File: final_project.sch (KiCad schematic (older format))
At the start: 0 parts

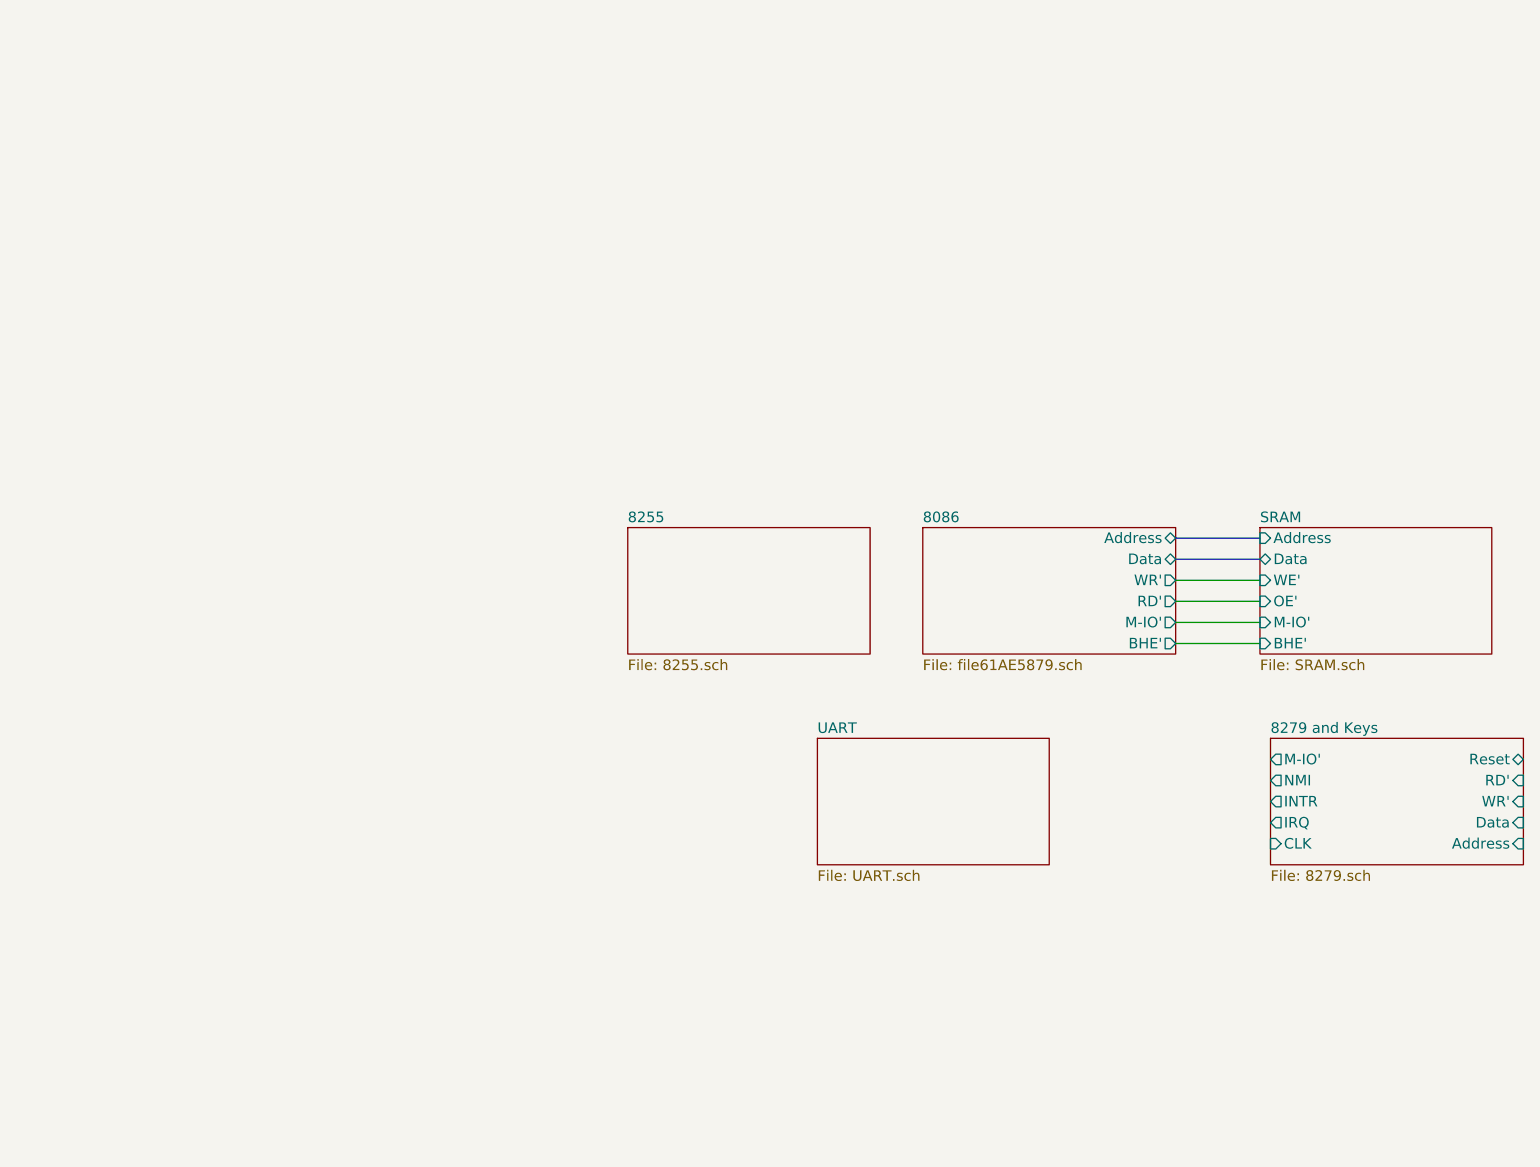
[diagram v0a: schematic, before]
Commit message: Merged 8254
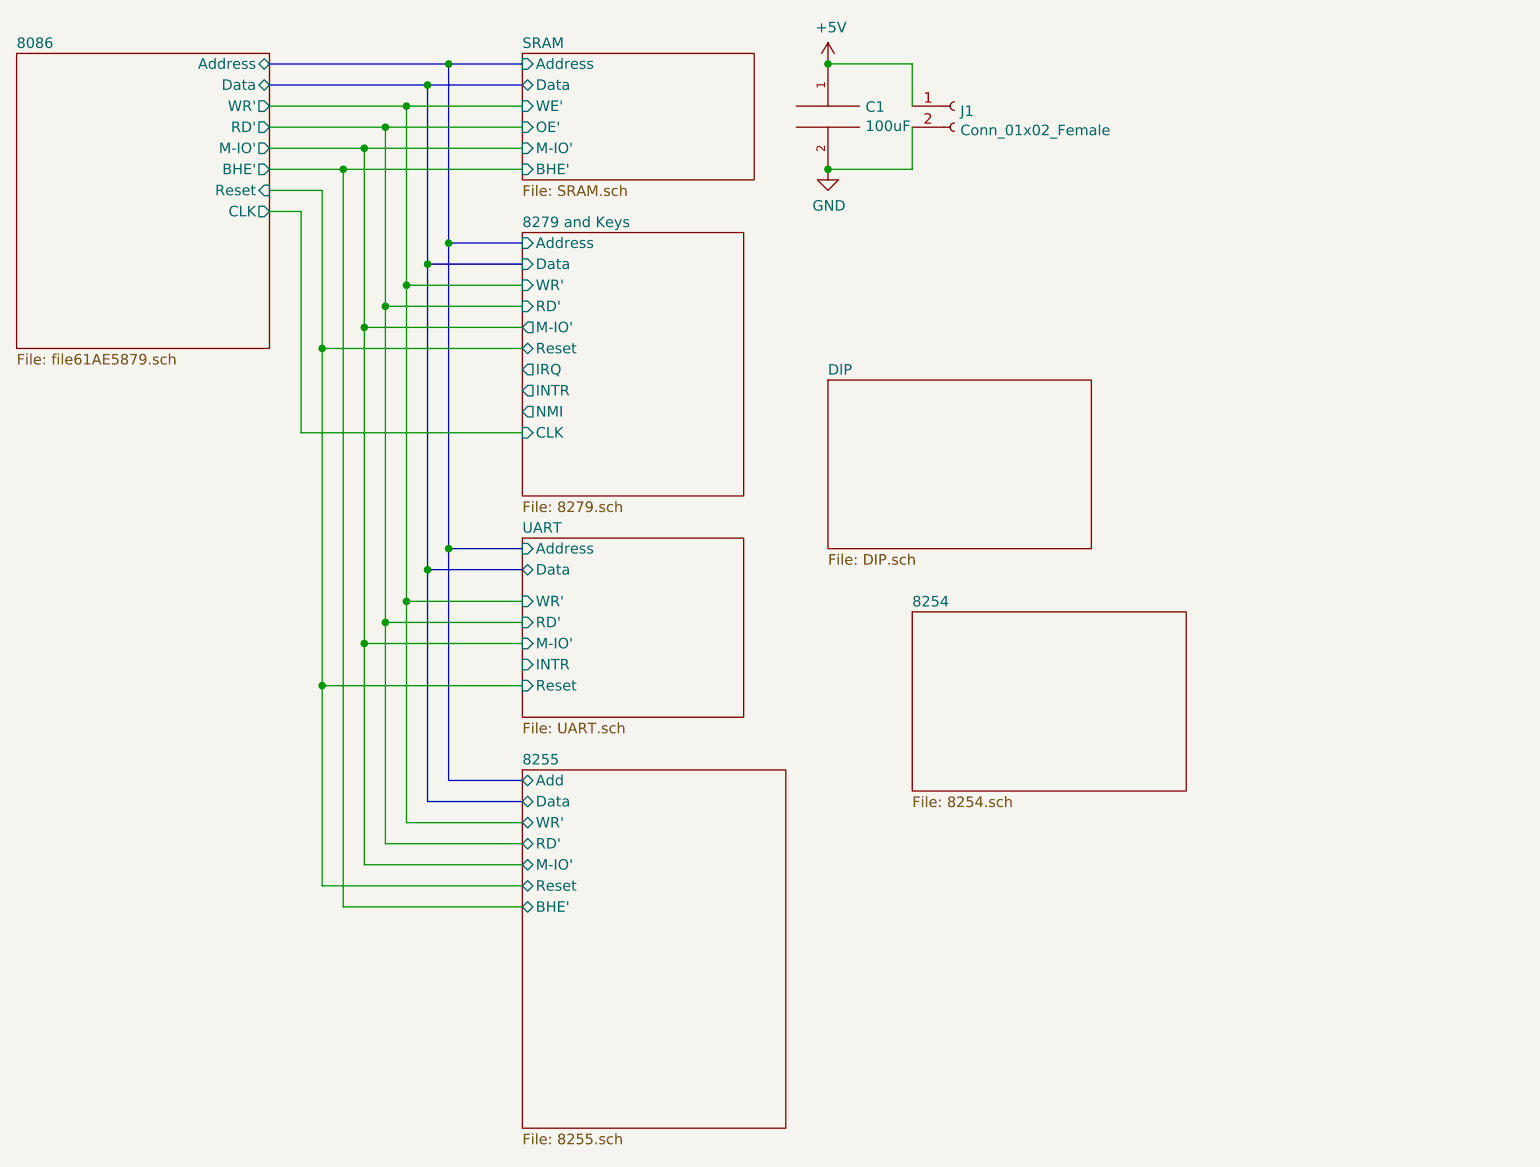
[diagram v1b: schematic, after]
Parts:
- added C1: 100uF, symbol pspice:C
- added J1: Conn_01x02_Female, symbol Connector:Conn_01x02_Female
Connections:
- new net +5V: C1.1, J1.1 (Pin_1)
- new net GND: C1.2, J1.2 (Pin_2)
